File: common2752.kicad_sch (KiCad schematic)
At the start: 12 parts, among them U30 LTC2752B, U31 OPA2189DGK, U35 LTC2752B, U36 OPA2189DGK

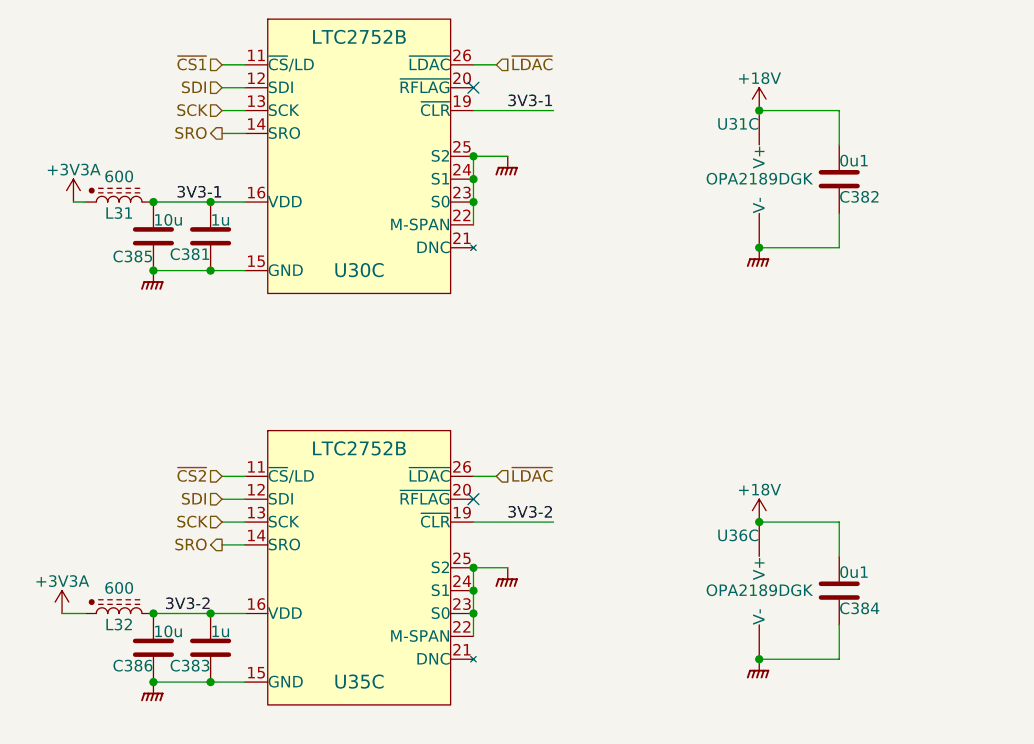
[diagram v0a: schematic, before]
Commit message: About to delete scan...
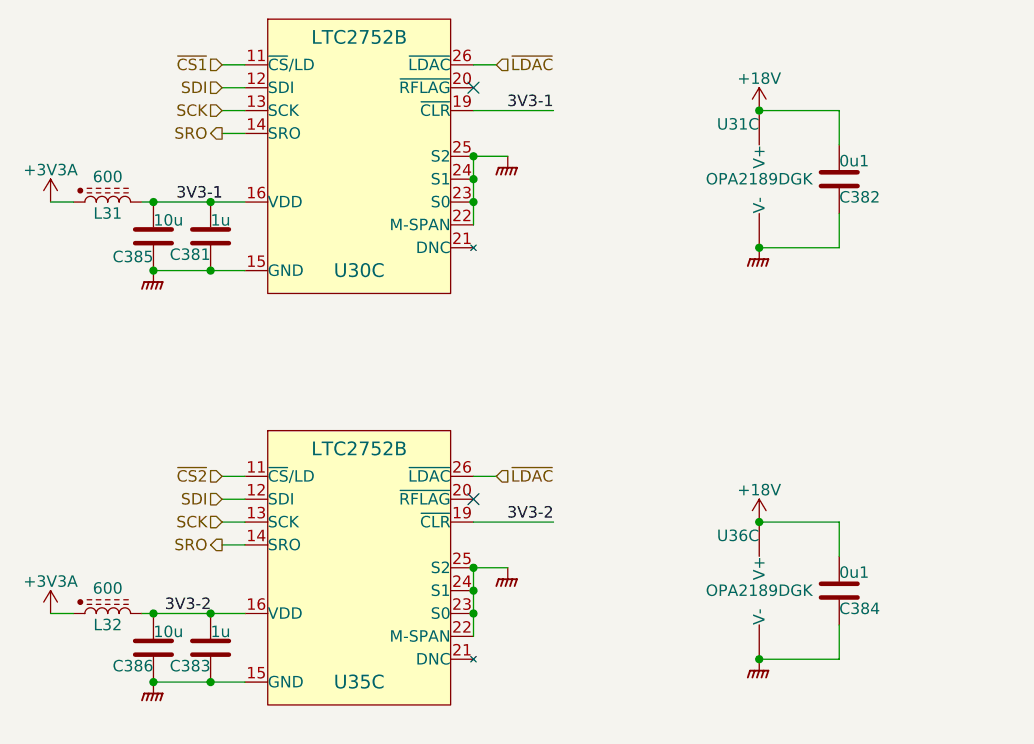
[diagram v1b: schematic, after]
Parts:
- U31, U36: Stock (none) -> 15
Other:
- moved on the sheet: L31, L32
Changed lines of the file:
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@@
+	(wire
+		(pts
+			(xy 41.91 71.12) (xy 43.18 71.12)
+		)
+		(stroke
+			(width 0)
+			(type default)
+		)
+	)
 	(wire
 		(pts
@@
 	(wire
 		(pts
-			(xy 33.02 116.84) (xy 35.56 116.84)
+			(xy 31.75 116.84) (xy 34.29 116.84)
 		)
 		(stroke
@@
 	(wire
 		(pts
-			(xy 34.29 71.12) (xy 35.56 71.12)
+			(xy 31.75 71.12) (xy 34.29 71.12)
 		)
 		(stroke
@@
 		(pts
 			(xy 119.38 106.68) (xy 110.49 106.68)
+		)
+		(stroke
+			(width 0)
+			(type default)
+		)
+	)
+	(wire
+		(pts
+			(xy 41.91 116.84) (xy 43.18 116.84)
 		)
 		(stroke
@@
 			)
 		)
+		(property "Stock" ""
+			(at 66.04 66.04 0)
+			(effects
+				(font
+					(size 1.27 1.27)
+				)
+				(hide yes)
+			)
+		)
 		(pin "18"
 		)
@@
 			)
 		)
+		(property "Stock" ""
+			(at 119.38 114.3 0)
+			(effects
+				(font
+					(size 1.27 1.27)
+				)
+				(hide yes)
+			)
+		)
 		(pin "2"
 		)
@@
 	(symbol
 		(lib_id "Parts:+3V3A")
-		(at 33.02 116.84 0)
+		(at 31.75 116.84 0)
 		(unit 1)
 		(exclude_from_sim no)
@@
 		(dnp no)
 		(property "Reference" "#PWR0732"
-			(at 33.02 120.65 0)
+			(at 31.75 120.65 0)
 			(effects
 				(font
@@
 		)
 		(property "Value" "+3V3A"
-			(at 33.02 113.284 0)
+			(at 31.75 113.284 0)
 			(do_not_autoplace yes)
 			(effects
@@
 		)
 		(property "Footprint" ""
-			(at 33.02 116.84 0)
+			(at 31.75 116.84 0)
 			(effects
 				(font
@@
 		)
 		(property "Datasheet" ""
-			(at 33.02 116.84 0)
+			(at 31.75 116.84 0)
 			(effects
 				(font
@@
 		)
 		(property "Description" "Power symbol creates a global label with name {dblquote}+3V3A{dblquote}"
-			(at 33.02 116.84 0)
+			(at 31.75 116.84 0)
 			(effects
 				(font
@@
 			)
 		)
+		(property "Stock" ""
+			(at 66.04 111.76 0)
+			(effects
+				(font
+					(size 1.27 1.27)
+				)
+				(hide yes)
+			)
+		)
 		(pin "18"
 		)
@@
 	(symbol
 		(lib_id "Parts:L_Ferrite_Power")
-		(at 39.37 116.84 90)
+		(at 38.1 116.84 90)
 		(unit 1)
 		(exclude_from_sim no)
@@
 		(dnp no)
 		(property "Reference" "L32"
-			(at 39.37 118.11 90)
+			(at 38.1 118.11 90)
 			(effects
 				(font
@@
 		)
 		(property "Value" "600"
-			(at 39.37 114.046 90)
+			(at 38.1 114.046 90)
 			(effects
 				(font
@@
 		)
 		(property "Footprint" "Inductor_SMD:L_0603_1608Metric"
-			(at 39.37 116.84 0)
+			(at 38.1 116.84 0)
 			(effects
 				(font
@@
 		)
 		(property "Datasheet" "200mA / 450mΩ"
-			(at 39.37 116.84 0)
+			(at 38.1 116.84 0)
 			(effects
 				(font
@@
 		)
 		(property "Description" "Inductor with ferrite core"
-			(at 39.37 116.84 0)
+			(at 38.1 116.84 0)
 			(effects
 				(font
@@
 		)
 		(property "LCSC" "C1002"
-			(at 39.37 116.84 90)
+			(at 38.1 116.84 90)
+			(effects
+				(font
+					(size 1.27 1.27)
+				)
+				(hide yes)
+			)
+		)
+		(property "Stock" ""
+			(at 38.1 116.84 90)
 			(effects
 				(font
@@
 	(symbol
 		(lib_id "Parts:L_Ferrite_Power")
-		(at 39.37 71.12 90)
+		(at 38.1 71.12 90)
 		(unit 1)
 		(exclude_from_sim no)
@@
 		(dnp no)
 		(property "Reference" "L31"
-			(at 39.37 72.39 90)
+			(at 38.1 72.39 90)
 			(effects
 				(font
@@
 		)
 		(property "Value" "600"
-			(at 39.37 68.326 90)
+			(at 38.1 68.326 90)
 			(effects
 				(font
@@
 		)
 		(property "Footprint" "Inductor_SMD:L_0603_1608Metric"
-			(at 39.37 71.12 0)
+			(at 38.1 71.12 0)
 			(effects
 				(font
@@
 		)
 		(property "Datasheet" "200mA / 450mΩ"
-			(at 39.37 71.12 0)
+			(at 38.1 71.12 0)
 			(effects
 				(font
@@
 		)
 		(property "Description" "Inductor with ferrite core"
-			(at 39.37 71.12 0)
+			(at 38.1 71.12 0)
 			(effects
 				(font
@@
 		)
 		(property "LCSC" "C1002"
-			(at 39.37 71.12 90)
+			(at 38.1 71.12 90)
+			(effects
+				(font
+					(size 1.27 1.27)
+				)
+				(hide yes)
+			)
+		)
+		(property "Stock" ""
+			(at 38.1 71.12 90)
 			(effects
 				(font
@@
 			)
 		)
+		(property "Stock" ""
+			(at 43.18 74.93 0)
+			(effects
+				(font
+					(size 1.27 1.27)
+				)
+				(hide yes)
+			)
+		)
 		(pin "1"
 		)
@@
 		)
 		(property "LCSC" "C307331"
+			(at 119.38 68.58 0)
+			(effects
+				(font
+					(size 1.27 1.27)
+				)
+				(hide yes)
+			)
+		)
+		(property "Stock" ""
 			(at 119.38 68.58 0)
 			(effects
@@
 			)
 		)
+		(property "Stock" "15"
+			(at 110.49 114.3 0)
+			(effects
+				(font
+					(size 1.27 1.27)
+				)
+				(hide yes)
+			)
+		)
 		(pin "1"
 		)
@@
 			)
 		)
+		(property "Stock" "15"
+			(at 110.49 68.58 0)
+			(effects
+				(font
+					(size 1.27 1.27)
+				)
+				(hide yes)
+			)
+		)
 		(pin "1"
 		)
@@
 			)
 		)
+		(property "Stock" ""
+			(at 49.53 74.93 0)
+			(effects
+				(font
+					(size 1.27 1.27)
+				)
+				(hide yes)
+			)
+		)
 		(pin "2"
 		)
@@
 			)
 		)
+		(property "Stock" ""
+			(at 43.18 120.65 0)
+			(effects
+				(font
+					(size 1.27 1.27)
+				)
+				(hide yes)
+			)
+		)
 		(pin "1"
 		)
@@
 	(symbol
 		(lib_id "Parts:+3V3A")
-		(at 34.29 71.12 0)
+		(at 31.75 71.12 0)
 		(unit 1)
 		(exclude_from_sim no)
@@
 		(dnp no)
 		(property "Reference" "#PWR0731"
-			(at 34.29 74.93 0)
+			(at 31.75 74.93 0)
 			(effects
 				(font
@@
 		)
 		(property "Value" "+3V3A"
-			(at 34.29 67.564 0)
+			(at 31.75 67.564 0)
 			(do_not_autoplace yes)
 			(effects
@@
 		)
 		(property "Footprint" ""
-			(at 34.29 71.12 0)
+			(at 31.75 71.12 0)
 			(effects
 				(font
@@
 		)
 		(property "Datasheet" ""
-			(at 34.29 71.12 0)
+			(at 31.75 71.12 0)
 			(effects
 				(font
@@
 		)
 		(property "Description" "Power symbol creates a global label with name {dblquote}+3V3A{dblquote}"
-			(at 34.29 71.12 0)
+			(at 31.75 71.12 0)
 			(effects
 				(font
@@
 			(at 49.53 120.65 0)
 			(effects
+				(font
+					(size 1.27 1.27)
+				)
+				(hide yes)
+			)
+		)
+		(property "Stock" ""
+			(at 49.53 120.65 0)
+			(effects

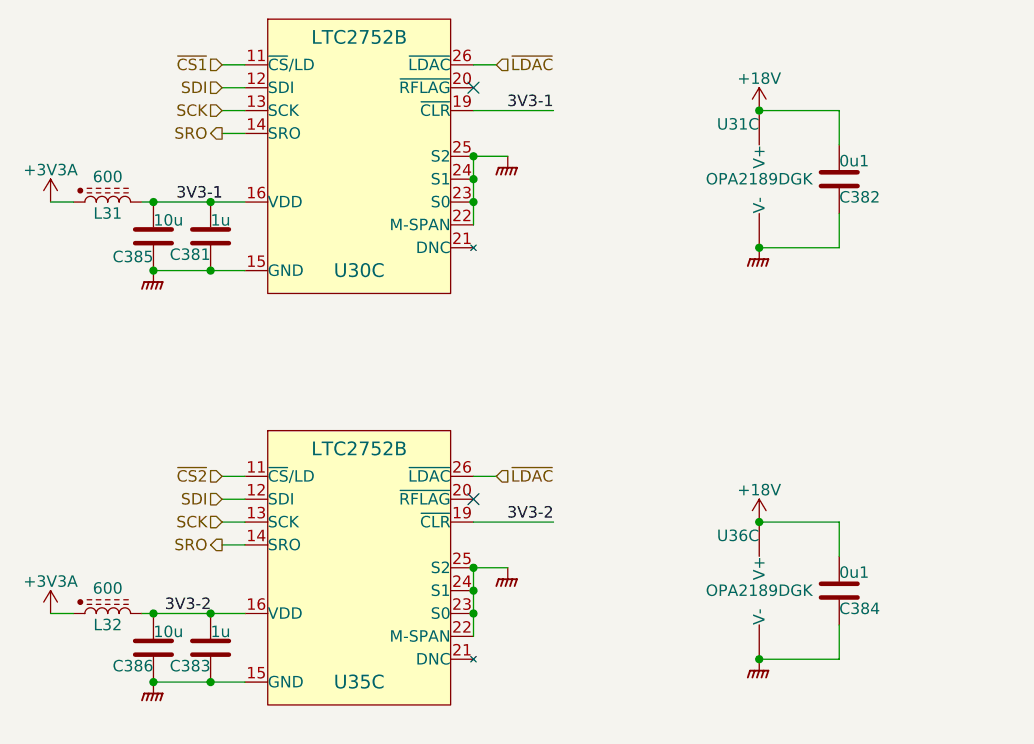
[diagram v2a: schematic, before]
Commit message: Most blocks there....
About to restore scan.
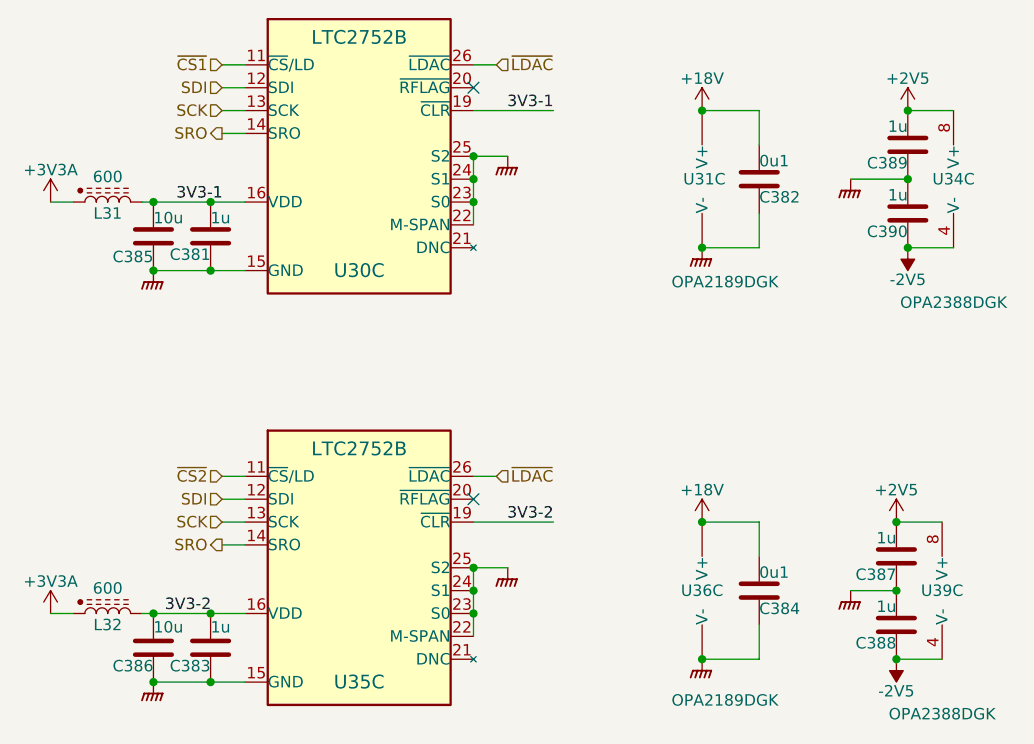
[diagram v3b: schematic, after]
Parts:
- added C387, C388, C389, C390: 1u, Capacitor_SMD:C_0402_1005Metric, symbol Device:C
- added U34, U39: OPA2388DGK, Parts:OPA2388, symbol Parts:OPA2388DGK
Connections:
- net GNDPWR: now also C387.2, C388.1, C389.2, C390.1
- new net +2V5: C387.1, C389.1, U34.8 (V+), U39.8 (V+)
- new net -2V5: C388.2, C390.2, U34.4 (V-), U39.4 (V-)
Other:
- moved on the sheet: C382, C384, U31C, U36C
